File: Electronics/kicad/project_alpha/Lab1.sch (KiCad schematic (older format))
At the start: 102 parts, among them J1 USB_OTG, J2 USB_B_Micro, J3 Conn_01x03_Female, J4 Conn_01x06_Female, J5 Conn_01x06_Female, SW1 SW_Push, SW2 SW_Push, SW3 SW_Push, SW4 SW_Push, SW5 SW_Push, U1 LM1117ADJ, U2 STM32F411RETx, U3 CS4270, U4 EADOGS102W-6, Y1 8.0MHz

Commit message: begin designing PCB
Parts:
- C1, C10, C12, C13, C14, C17, C2, C3, C4, C6, C7, C8, C9: symbol Lab1-rescue:C-Device -> Lab1-rescue:C-Device-Lab1-rescue
- C11, C5: symbol Lab1-rescue:CP-device -> Lab1-rescue:CP-device-Lab1-rescue
- C15: footprint Capacitor_SMD:C_Elec_6.3x7.7 -> Capacitor_SMD:CP_Elec_4x5.4; symbol Lab1-rescue:C-device -> Lab1-rescue:C-device-Lab1-rescue
- C16, C22, C23, C24, C25: symbol Lab1-rescue:C-device -> Lab1-rescue:C-device-Lab1-rescue
- C20, C21, C37, C38, C39, C40, C41: footprint Capacitor_SMD:CP_Elec_5x5.9 -> Capacitor_SMD:CP_Elec_4x5.4
- C28, C29: footprint Capacitor_SMD:C_Elec_6.3x7.7 -> Capacitor_SMD:C_0805_2012Metric_Pad1.15x1.40mm_HandSolder; symbol Lab1-rescue:C-device -> Lab1-rescue:C-device-Lab1-rescue
- J1: symbol Lab1-rescue:USB_OTG-Connector -> Lab1-rescue:USB_OTG-Connector-Lab1-rescue
- R1, R13, R14, R18, R19, R2, R20, R21, R3, R4: symbol Lab1-rescue:R-Device -> Lab1-rescue:R-Device-Lab1-rescue
- U1: symbol Library_Lab1:LM1117ADJ -> Lab1-rescue:LM1117ADJ-Library_Lab1
- U2: symbol Lab1-rescue:STM32F411RETx-MCU_ST_STM32F4 -> Lab1-rescue:STM32F411RETx-MCU_ST_STM32F4-Lab1-rescue
- U3: symbol Library_Lab1:CS4270 -> Lab1-rescue:CS4270-Library_Lab1
- U4: symbol Library_Lab1:EADOGS102W-6 -> Lab1-rescue:EADOGS102W-6-Library_Lab1
- Y1: symbol Lab1-rescue:Crystal-Device -> Lab1-rescue:Crystal-Device-Lab1-rescue
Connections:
- wire segments 377 -> 376

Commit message: update PCB, not done yet
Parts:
- removed C22: 47u, Capacitor_SMD:C_Elec_6.3x7.7, symbol Lab1-rescue:C-device-Lab1-rescue
- removed C37, C38: 1u, Capacitor_SMD:CP_Elec_4x5.4, symbol Device:CP
- added C22: 47u, Capacitor_SMD:CP_Elec_4x5.4, symbol Lab1-rescue:CP-Device
- added C37, C38: 1u, Capacitor_SMD:C_0805_2012Metric_Pad1.15x1.40mm_HandSolder, symbol Lab1-rescue:C-device-Lab1-rescue
- C18, C19, C26, C27, C32, C33, C34, C35, C36, C42: symbol Device:C -> Lab1-rescue:C-Device
- C20, C21, C30, C31, C39, C40, C41: symbol Device:CP -> Lab1-rescue:CP-Device
- C23: value 47u -> 10u
- D1, D2, D3, D4: symbol Device:LED -> Lab1-rescue:LED-Device
- H1, H2: symbol Mechanical:MountingHole_Pad -> Lab1-rescue:MountingHole_Pad-Mechanical
- J2: symbol Connector:USB_B_Micro -> Lab1-rescue:USB_B_Micro-Connector
- J3: symbol Connector:Conn_01x03_Female -> Lab1-rescue:Conn_01x03_Female-Connector
- J4, J5: symbol Connector:Conn_01x06_Female -> Lab1-rescue:Conn_01x06_Female-Connector
- R10, R11, R12, R15, R16, R17, R22, R23, R24, R25, R26, R27, R28, R29, R30, R31, R32, R33, R34, R35, R36, R5, R6, R7, R8, R9: symbol Device:R -> Lab1-rescue:R-Device
- RV1, RV2, RV3: symbol Device:R_POT -> Lab1-rescue:R_POT-Device
- SW1, SW2, SW3, SW4, SW5: symbol Switch:SW_Push -> Lab1-rescue:SW_Push-Switch
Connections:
- net +3V3: now also C38.1
- net +5V: now also C37.2
- net GNDA: now also C22.2, C37.1
- net GNDD: now also C38.2
- net at C24.1, U3.18 (FILT+): now also C22.1

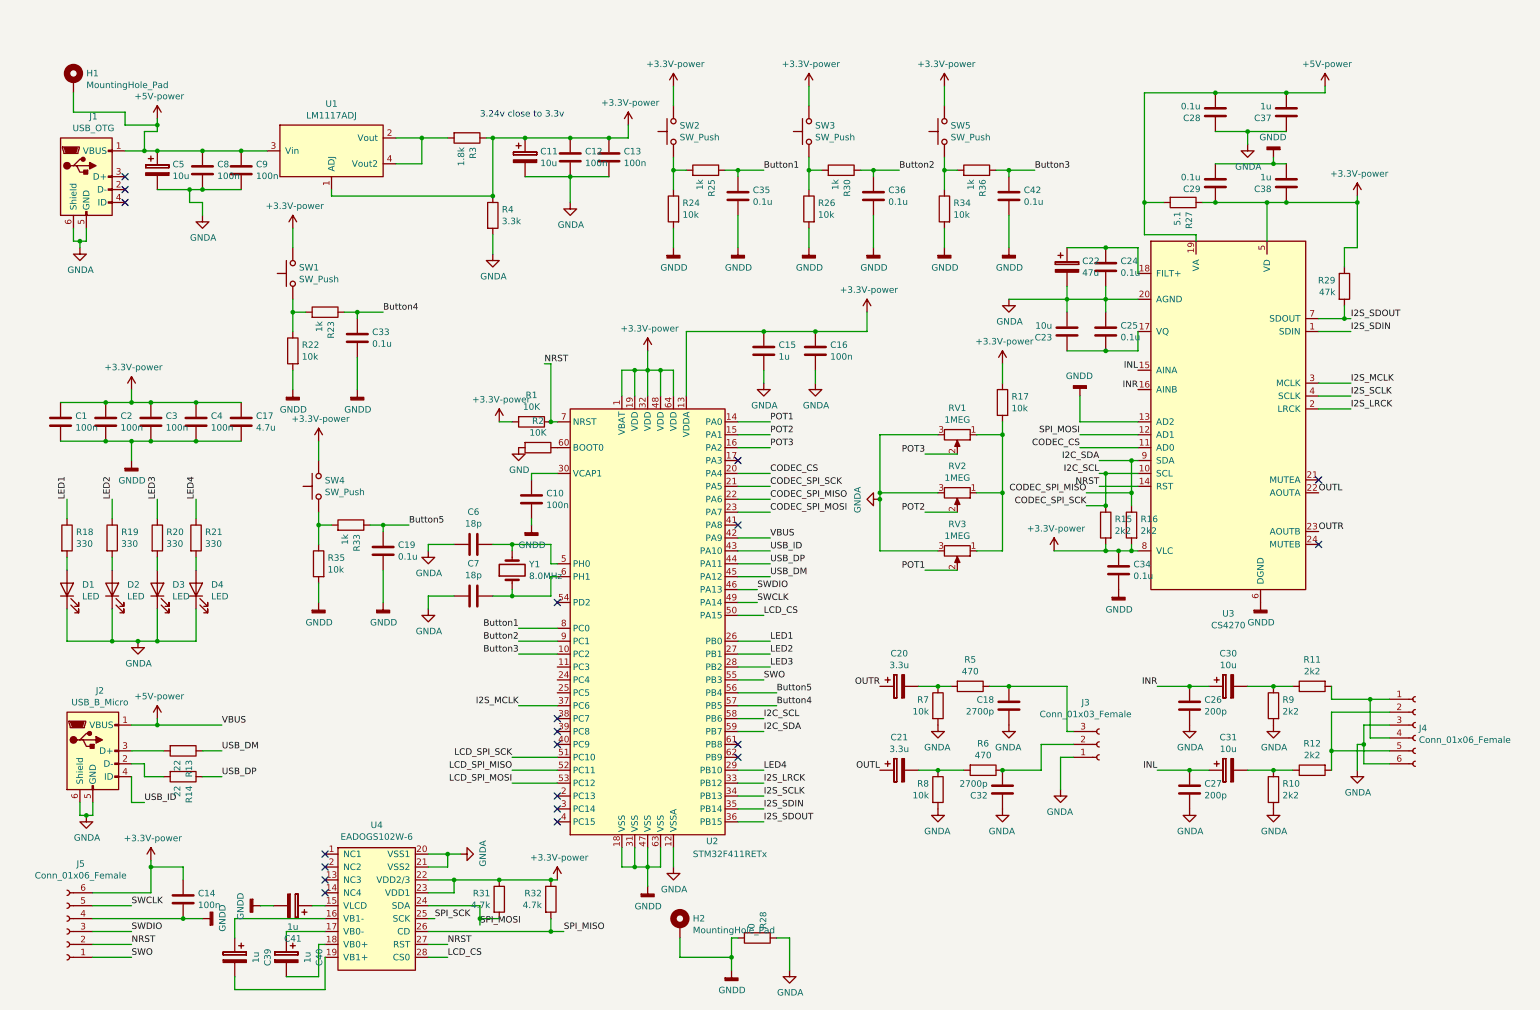
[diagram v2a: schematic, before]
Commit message: update PCB
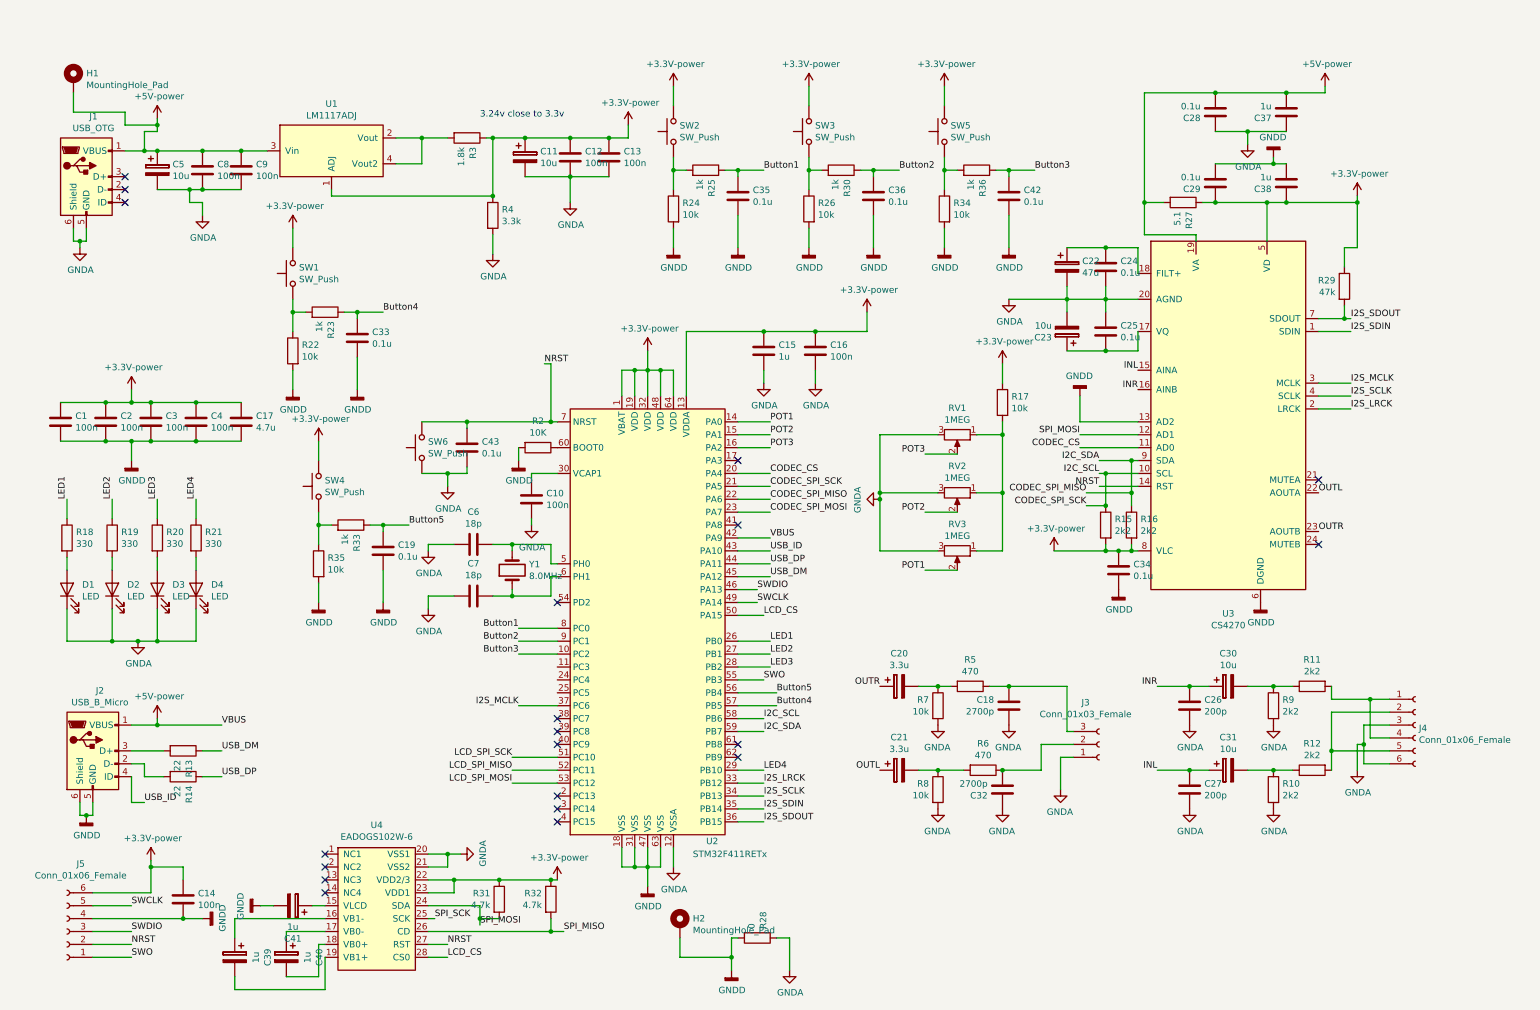
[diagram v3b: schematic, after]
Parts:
- removed C23: 10u, Capacitor_SMD:C_Elec_6.3x7.7, symbol Lab1-rescue:C-device-Lab1-rescue
- removed R1: 10K, Resistor_SMD:R_0805_2012Metric_Pad1.15x1.40mm_HandSolder, symbol Lab1-rescue:R-Device-Lab1-rescue
- added C23: 10u, Capacitor_SMD:CP_Elec_5x5.4, symbol Lab1-rescue:CP-Device
- added C43: 0.1u, Capacitor_SMD:C_0805_2012Metric_Pad1.15x1.40mm_HandSolder, symbol Lab1-rescue:C-device-Lab1-rescue
- added SW6: SW_Push, Button_Switch_SMD:SW_SPST_B3S-1000, symbol Lab1-rescue:SW_Push-Switch
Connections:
- net GND is gone; now on net GNDD: R2.2
- net GNDA: now also C10.2, C23.2, C43.2, SW6.1; no longer J2.5 (GND), J2.6 (Shield)
- net GNDD: now also J2.5 (GND), J2.6 (Shield); no longer C10.2
- net NRST: now also C43.1, SW6.2
- net at C25.2, U3.17 (VQ): now also C23.1
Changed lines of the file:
@@
 Comment4 ""
 $EndDescr
-$Comp
-L Lab1-rescue:R-Device-Lab1-rescue R1
-U 1 1 5C49EC6C
-P 4250 3300
-F 0 "R1" V 4043 3300 50  0000 C CNN
-F 1 "10K" V 4134 3300 50  0000 C CNN
-F 2 "Resistor_SMD:R_0805_2012Metric_Pad1.15x1.40mm_HandSolder" V 4180 3300 50  0001 C CNN
-F 3 "~" H 4250 3300 50  0001 C CNN
-	1    4250 3300
-	0    1    1    0
-$EndComp
 Wire Wire Line
 	4400 3300 4450 3300
@@
 $EndComp
 $Comp
-L Lab1-rescue:GND-power-Lab1-rescue #PWR09
-U 1 1 5C4A10A9
-P 4150 3500
-F 0 "#PWR09" H 4150 3250 50  0001 C CNN
-F 1 "GND" H 4155 3327 50  0000 C CNN
-F 2 "" H 4150 3500 50  0001 C CNN
-F 3 "" H 4150 3500 50  0001 C CNN
-	1    4150 3500
-	1    0    0    -1
-$EndComp
-$Comp
 L Lab1-rescue:Crystal-Device-Lab1-rescue Y1
 U 1 1 5C4A1143
@@
 	3450 4650 3650 4650
 Wire Wire Line
-	4100 3300 4000 3300
-Wire Wire Line
 	1300 6950 1300 6750
 Wire Wire Line
@@
 Wire Wire Line
 	4400 2850 4400 3300
-Connection ~ 4400 3300
 Text Label 4350 2850 0    50   ~ 0
 NRST
@@
 F 3 "" H 1150 3050 50  0001 C CNN
 	1    1150 3050
-	1    0    0    -1
-$EndComp
-$Comp
-L Lab1-rescue:+3.3V-power-Lab1-rescue #PWR0106
-U 1 1 5C4C0FE6
-P 4000 3300
-F 0 "#PWR0106" H 4000 3150 50  0001 C CNN
-F 1 "+3.3V-power" H 4015 3473 50  0000 C CNN
-F 2 "" H 4000 3300 50  0001 C CNN
-F 3 "" H 4000 3300 50  0001 C CNN
-	1    4000 3300
 	1    0    0    -1
 $EndComp
@@
 Wire Wire Line
 	6850 2600 6850 2450
-$Comp
-L Lab1-rescue:C-device-Lab1-rescue C23
-U 1 1 5C66D78F
-P 8400 2600
-F 0 "C23" H 8515 2646 50  0000 L CNN
-F 1 "10u" H 8515 2555 50  0000 L CNN
-F 2 "Capacitor_SMD:C_Elec_6.3x7.7" H 8438 2450 50  0001 C CNN
-F 3 "~" H 8400 2600 50  0001 C CNN
-	1    8400 2600
-	-1   0    0    1
-$EndComp
 $Comp
 L Lab1-rescue:C-device-Lab1-rescue C25
@@
 $EndComp
 $Comp
-L Lab1-rescue:GNDA-power #PWR07
-U 1 1 5C586751
-P 3450 4300
-F 0 "#PWR07" H 3450 4050 50  0001 C CNN
-F 1 "GNDA" H 3455 4127 50  0000 C CNN
-F 2 "" H 3450 4300 50  0001 C CNN
-F 3 "" H 3450 4300 50  0001 C CNN
-	1    3450 4300
-	1    0    0    -1
-$EndComp
-$Comp
-L Lab1-rescue:GNDA-power #PWR012
-U 1 1 5C5867C7
-P 3450 4750
-F 0 "#PWR012" H 3450 4500 50  0001 C CNN
-F 1 "GNDA" H 3455 4577 50  0000 C CNN
-F 2 "" H 3450 4750 50  0001 C CNN
-F 3 "" H 3450 4750 50  0001 C CNN
-	1    3450 4750
-	1    0    0    -1
-$EndComp
-$Comp
 L Lab1-rescue:GNDA-power #PWR018
 U 1 1 5C586838
@@
 Wire Wire Line
 	1850 5650 1350 5650
-$Comp
-L Lab1-rescue:GNDA-power #PWR05
-U 1 1 5C6487AC
-P 800 6350
-F 0 "#PWR05" H 800 6100 50  0001 C CNN
-F 1 "GNDA" H 805 6177 50  0000 C CNN
-F 2 "" H 800 6350 50  0001 C CNN
-F 3 "" H 800 6350 50  0001 C CNN
-	1    800  6350
-	1    0    0    -1
-$EndComp
 Wire Wire Line
 	750  6250 750  6350
 Wire Wire Line
-	750  6350 800  6350
-Wire Wire Line
 	850  6250 850  6350
-Wire Wire Line
-	850  6350 800  6350
-Connection ~ 800  6350
 Wire Wire Line
 	1150 5950 1250 5950
@@
 NoConn ~ 2650 6750
 NoConn ~ 2650 6650
-$Comp
-L Lab1-rescue:GNDD-power #PWR0109
-U 1 1 5CAE84EF
-P 4250 4100
-F 0 "#PWR0109" H 4250 3850 50  0001 C CNN
-F 1 "GNDD" H 4254 3945 50  0000 C CNN
-F 2 "" H 4250 4100 50  0001 C CNN
-F 3 "" H 4250 4100 50  0001 C CNN
-	1    4250 4100
-	1    0    0    -1
-$EndComp
 Text Label 8500 3400 2    50   ~ 0
 SPI_MOSI
@@
 Wire Wire Line
 	10100 1600 10650 1600
+$Comp
+L Lab1-rescue:GNDA-power #PWR09
+U 1 1 5C679FB9
+P 3450 4750
+F 0 "#PWR09" H 3450 4500 50  0001 C CNN
+F 1 "GNDA" H 3455 4577 50  0000 C CNN
+F 2 "" H 3450 4750 50  0001 C CNN
+F 3 "" H 3450 4750 50  0001 C CNN
+	1    3450 4750
+	1    0    0    -1
+$EndComp
+$Comp
+L Lab1-rescue:GNDA-power #PWR07
+U 1 1 5C67A08E
+P 3450 4300
+F 0 "#PWR07" H 3450 4050 50  0001 C CNN
+F 1 "GNDA" H 3455 4127 50  0000 C CNN
+F 2 "" H 3450 4300 50  0001 C CNN
+F 3 "" H 3450 4300 50  0001 C CNN
+	1    3450 4300
+	1    0    0    -1
+$EndComp
+$Comp
+L Lab1-rescue:GNDA-power #PWR057
+U 1 1 5C67A163
+P 4250 4100
+F 0 "#PWR057" H 4250 3850 50  0001 C CNN
+F 1 "GNDA" H 4255 3927 50  0000 C CNN
+F 2 "" H 4250 4100 50  0001 C CNN
+F 3 "" H 4250 4100 50  0001 C CNN
+	1    4250 4100
+	1    0    0    -1
+$EndComp
+$Comp
+L Lab1-rescue:SW_Push-Switch SW6
+U 1 1 5C67A367
+P 3400 3500
+F 0 "SW6" V 3446 3452 50  0000 R CNN
+F 1 "SW_Push" V 3355 3452 50  0000 R CNN
+F 2 "Button_Switch_SMD:SW_SPST_B3S-1000" H 3400 3700 50  0001 C CNN
+F 3 "" H 3400 3700 50  0001 C CNN
+	1    3400 3500
+	0    -1   -1   0
+$EndComp
+$Comp
+L Lab1-rescue:C-device-Lab1-rescue C43
+U 1 1 5C67A4A5
+P 3750 3500
+F 0 "C43" H 3865 3546 50  0000 L CNN
+F 1 "0.1u" H 3865 3455 50  0000 L CNN
+F 2 "Capacitor_SMD:C_0805_2012Metric_Pad1.15x1.40mm_HandSolder" H 3788 3350 50  0001 C CNN
+F 3 "~" H 3750 3500 50  0001 C CNN
+	1    3750 3500
+	1    0    0    -1
+$EndComp
+$Comp
+L Lab1-rescue:GNDD-power #PWR056
+U 1 1 5C6A077E
+P 4150 3600
+F 0 "#PWR056" H 4150 3350 50  0001 C CNN
+F 1 "GNDD" H 4154 3445 50  0000 C CNN
+F 2 "" H 4150 3600 50  0001 C CNN
+F 3 "" H 4150 3600 50  0001 C CNN
+	1    4150 3600
+	1    0    0    -1
+$EndComp
+Wire Wire Line
+	4150 3500 4150 3600
+$Comp
+L Lab1-rescue:GNDA-power #PWR012
+U 1 1 5C6C690F
+P 3600 3800
+F 0 "#PWR012" H 3600 3550 50  0001 C CNN
+F 1 "GNDA" H 3605 3627 50  0000 C CNN
+F 2 "" H 3600 3800 50  0001 C CNN
+F 3 "" H 3600 3800 50  0001 C CNN
+	1    3600 3800
+	1    0    0    -1
+$EndComp
+Wire Wire Line
+	3400 3700 3600 3700
+Wire Wire Line
+	3600 3700 3600 3800
+Wire Wire Line
+	3750 3650 3750 3700
+Wire Wire Line
+	3750 3700 3600 3700
+Connection ~ 3600 3700
+Wire Wire Line
+	3400 3300 3750 3300
+Connection ~ 4400 3300
+Wire Wire Line
+	3750 3350 3750 3300
+Connection ~ 3750 3300
+Wire Wire Line
+	3750 3300 4400 3300
+Wire Wire Line
+	750  6350 800  6350
+$Comp
+L Lab1-rescue:GNDD-power #PWR0106
+U 1 1 5C76A089
+P 800 6350
+F 0 "#PWR0106" H 800 6100 50  0001 C CNN
+F 1 "GNDD" H 804 6195 50  0000 C CNN
+F 2 "" H 800 6350 50  0001 C CNN
+F 3 "" H 800 6350 50  0001 C CNN
+	1    800  6350
+	1    0    0    -1
+$EndComp
+Connection ~ 800  6350
+Wire Wire Line
+	800  6350 850  6350
+$Comp
+L Lab1-rescue:CP-Device C23
+U 1 1 5C772344
+P 8400 2600
+F 0 "C23" H 8518 2646 50  0000 L CNN
+F 1 "10u" H 8518 2555 50  0000 L CNN
+F 2 "Capacitor_SMD:CP_Elec_5x5.4" H 8438 2450 50  0001 C CNN
+F 3 "" H 8400 2600 50  0001 C CNN
+	1    8400 2600
+	-1   0    0    1
+$EndComp
 $EndSCHEMATC

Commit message: update PCB
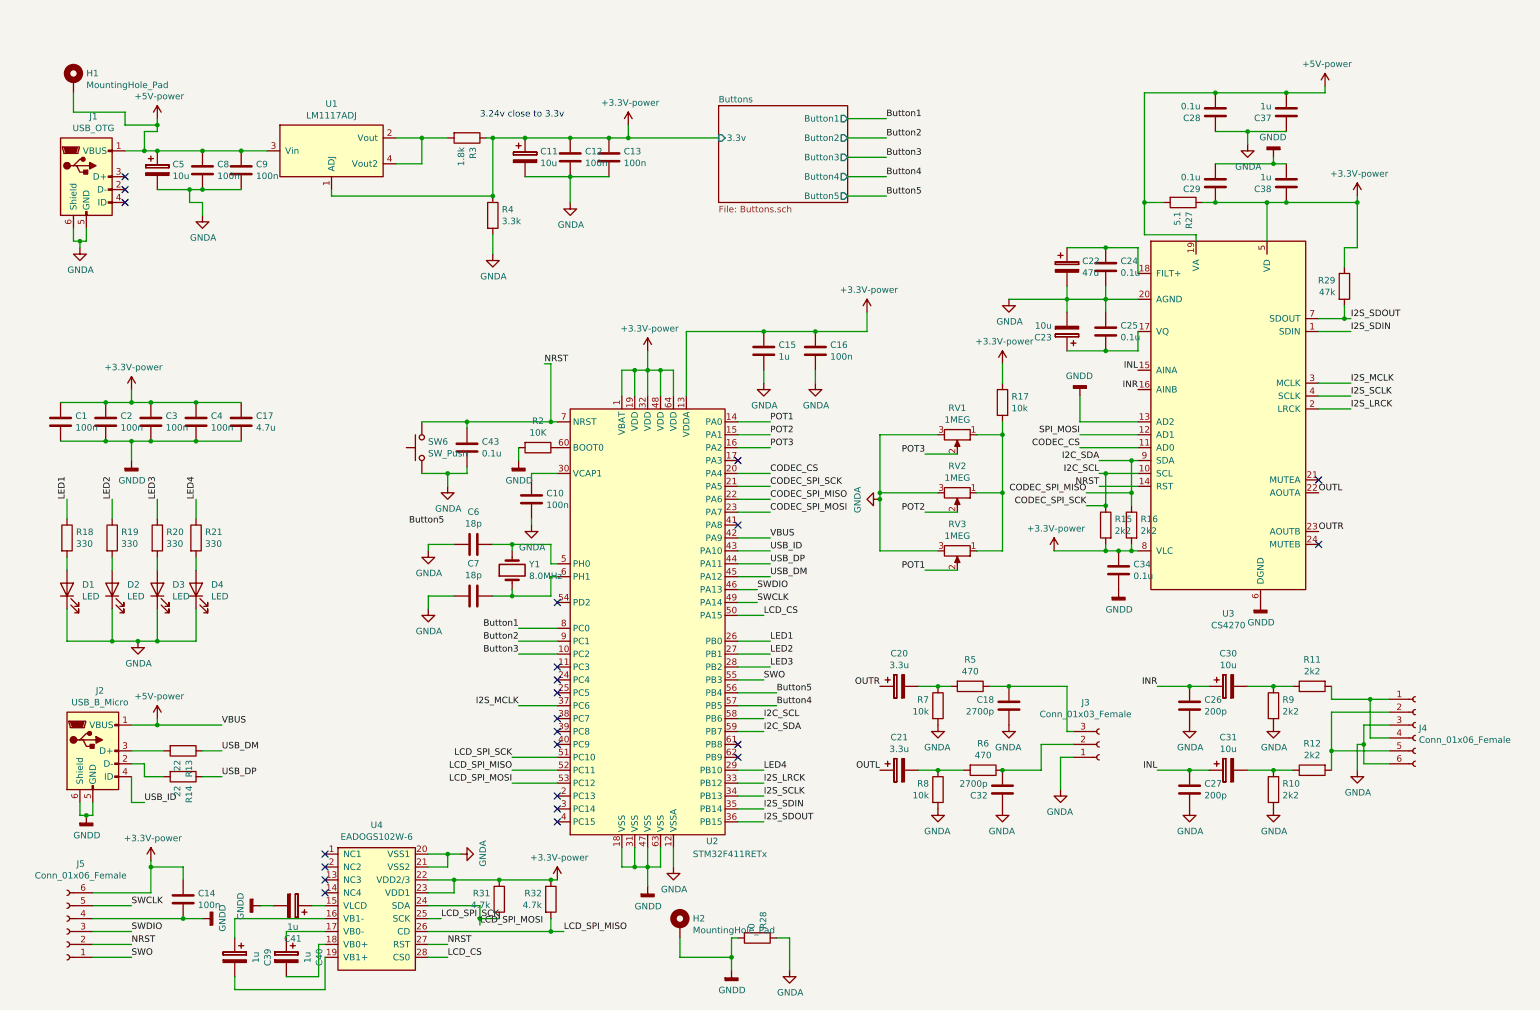
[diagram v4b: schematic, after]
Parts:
- removed C19, C33, C35, C36, C42: 0.1u, Capacitor_SMD:C_0805_2012Metric_Pad1.15x1.40mm_HandSolder, symbol Lab1-rescue:C-Device
- removed R22, R24, R26, R34, R35: 10k, Resistor_SMD:R_0805_2012Metric_Pad1.15x1.40mm_HandSolder, symbol Lab1-rescue:R-Device
- removed R23, R25, R30, R33, R36: 1k, Resistor_SMD:R_0805_2012Metric_Pad1.15x1.40mm_HandSolder, symbol Lab1-rescue:R-Device
- removed SW1, SW2, SW3, SW4, SW5: SW_Push, Button_Switch_SMD:SW_SPST_B3S-1000, symbol Lab1-rescue:SW_Push-Switch
- C15: footprint Capacitor_SMD:CP_Elec_4x5.4 -> Capacitor_SMD:C_0805_2012Metric_Pad1.15x1.40mm_HandSolder
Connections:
- net SPI_MISO is gone; now on net LCD_SPI_MISO: R32.2, U4.26 (CD)
- net SPI_SCK is gone; now on net LCD_SPI_SCK: U4.25 (SCK)
- net LCD_SPI_MOSI: now also R31.2, U4.24 (SDA)
- net SPI_MOSI: no longer R31.2, U4.24 (SDA)
- no-connect marks 20 -> 23
